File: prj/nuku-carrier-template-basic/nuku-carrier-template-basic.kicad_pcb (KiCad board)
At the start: 4 copper layers, 100 x 60 mm, 93 parts, among them J1 DF40HC(4.0)-90DS-0.4V, J2 DF40HC(4.0)-90DS-0.4V, J3 DF40HC(4.0)-90DS-0.4V, J4 DF40HC(4.0)-90DS-0.4V, J5 USB_C_Receptacle_USB2.0_16P, J6 TC2050, J7 PMOD_A, J8 PMOD_B, SW1 PROG, SW2 RESET, U1 AP61302, U10 SRV05-4, U2 SRV05-4, U3 M93C56-WDW6TP, U4 FT2232HQ, U5 IS25LP064A, U6 OT3225100MJBA4SL, U7 SRV05-4, U8 SRV05-4, U9 SRV05-4, Y1 12 MHz

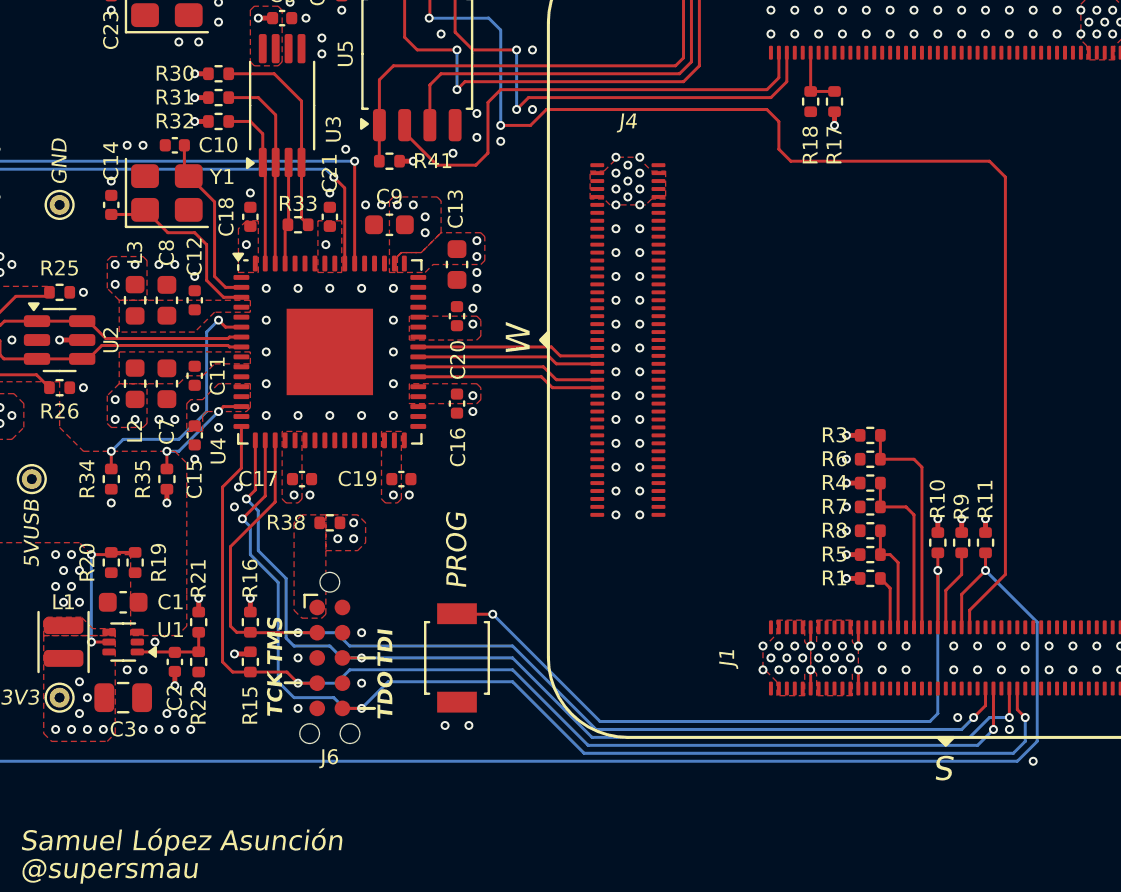
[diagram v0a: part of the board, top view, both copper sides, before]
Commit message: Finish bridgeless template
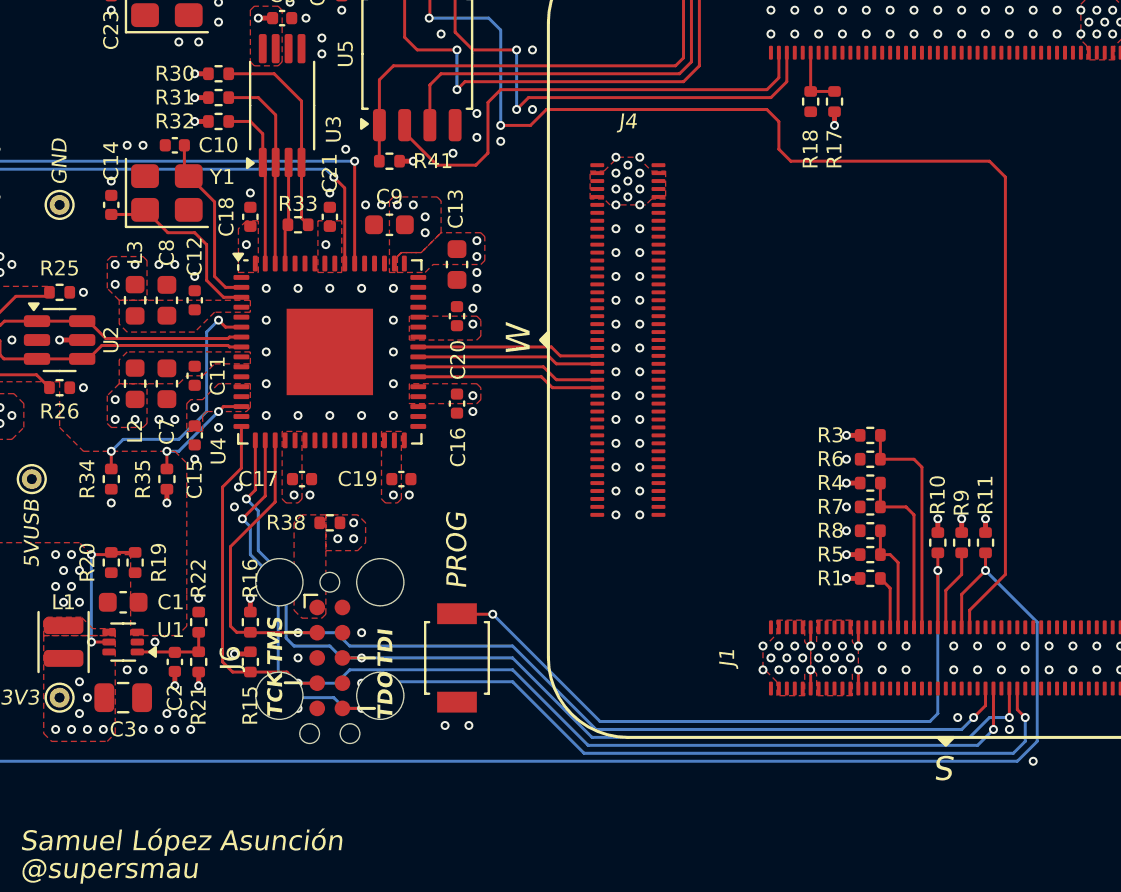
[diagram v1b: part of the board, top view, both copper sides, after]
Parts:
- J6: footprint Connector:Tag-Connect_TC2050-IDC-NL_2x05_P1.27mm_Vertical -> Connector:Tag-Connect_TC2050-IDC-FP_2x05_P1.27mm_Vertical
- moved R21 2.00 mm to (110.9, 121.2), turned to -90 degrees
- moved R22 2.00 mm to (110.9, 119.2), turned to -90 degrees
